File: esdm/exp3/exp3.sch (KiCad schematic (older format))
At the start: 1 part

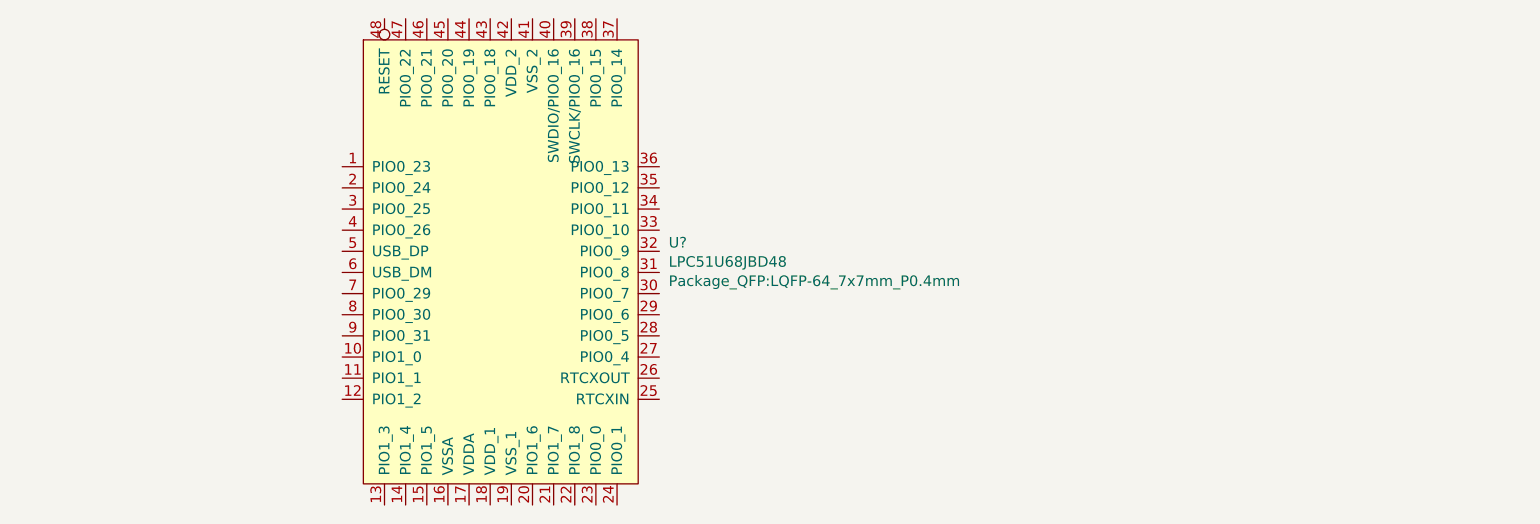
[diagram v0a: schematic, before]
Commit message: corrected exp 3
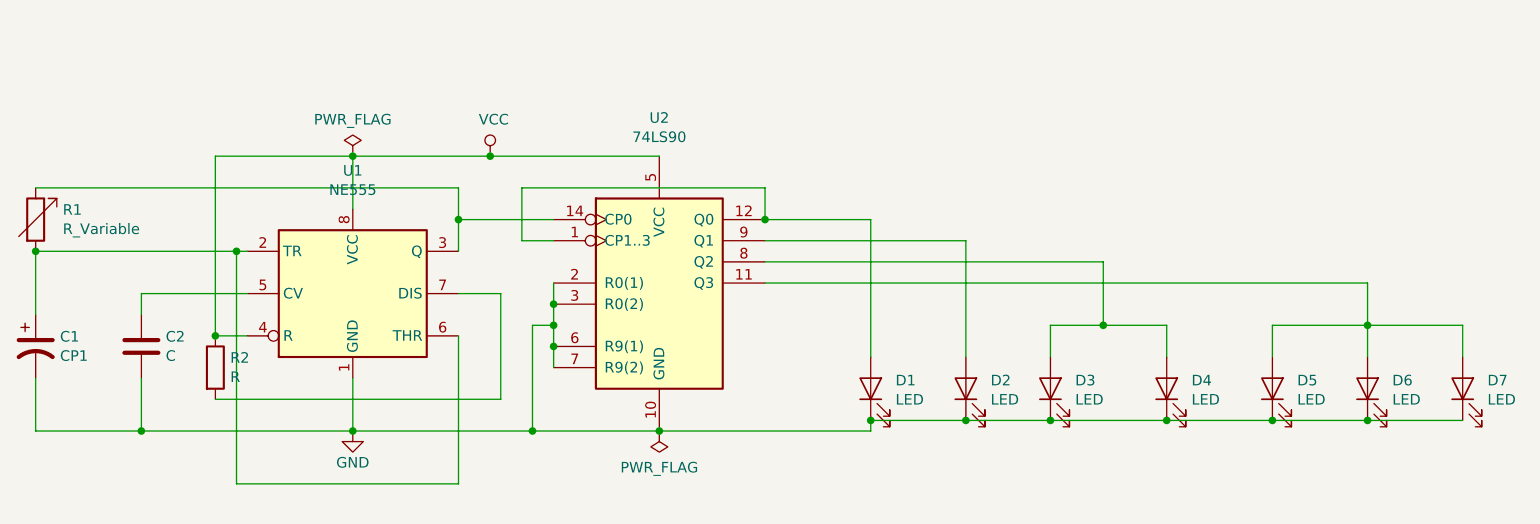
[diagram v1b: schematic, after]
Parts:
- removed U?: LPC51U68JBD48, Package_QFP:LQFP-64_7x7mm_P0.4mm, symbol LPC51U68JBD48:LPC51U68JBD48
- added C1: CP1, symbol Device:CP1
- added C2: C, symbol Device:C
- added D1, D2, D3, D4, D5, D6, D7: LED, symbol Device:LED
- added R1: R_Variable, symbol Device:R_Variable
- added R2: R, symbol Device:R
- added U1: NE555, symbol Timer:NE555
- added U2: 74LS90, symbol 74xx:74LS90
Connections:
- new net: D1.2 (A), U2.1 (CP1..3), U2.12 (Q0)
- new net: D5.2 (A), D6.2 (A), D7.2 (A), U2.11 (Q3)
- new net: R1.1, U1.3 (Q), U2.14 (CP0)
- new net: D3.2 (A), D4.2 (A), U2.8 (Q2)
- new net: D2.2 (A), U2.9 (Q1)
- new net: R2.2, U1.7 (DIS)
- new net: C1.1, R1.2, U1.2 (TR), U1.6 (THR)
- new net: C2.1, U1.5 (CV)
- new net GND: C1.2, C2.2, D1.1 (K), D2.1 (K), D3.1 (K), D4.1 (K), D5.1 (K), D6.1 (K), D7.1 (K), U1.1 (GND), U2.10 (GND), U2.2 (R0(1)), U2.3 (R0(2)), U2.6 (R9(1)), U2.7 (R9(2))
- new net VCC: R2.1, U1.4 (R), U1.8 (VCC), U2.5 (VCC)
